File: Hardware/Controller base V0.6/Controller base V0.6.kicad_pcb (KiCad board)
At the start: 2 copper layers, 30.1 x 48.9 mm, 23 parts, among them J1 USB_C_Receptacle_USB2.0_16P, J7 Conn_02x10_Counter_Clockwise, J8 Conn_02x10_Counter_Clockwise, SW4 SW_Push, U1 AZ1117CH-3.3TRG1, U2 ESP32-S3-WROOM-1U-N4

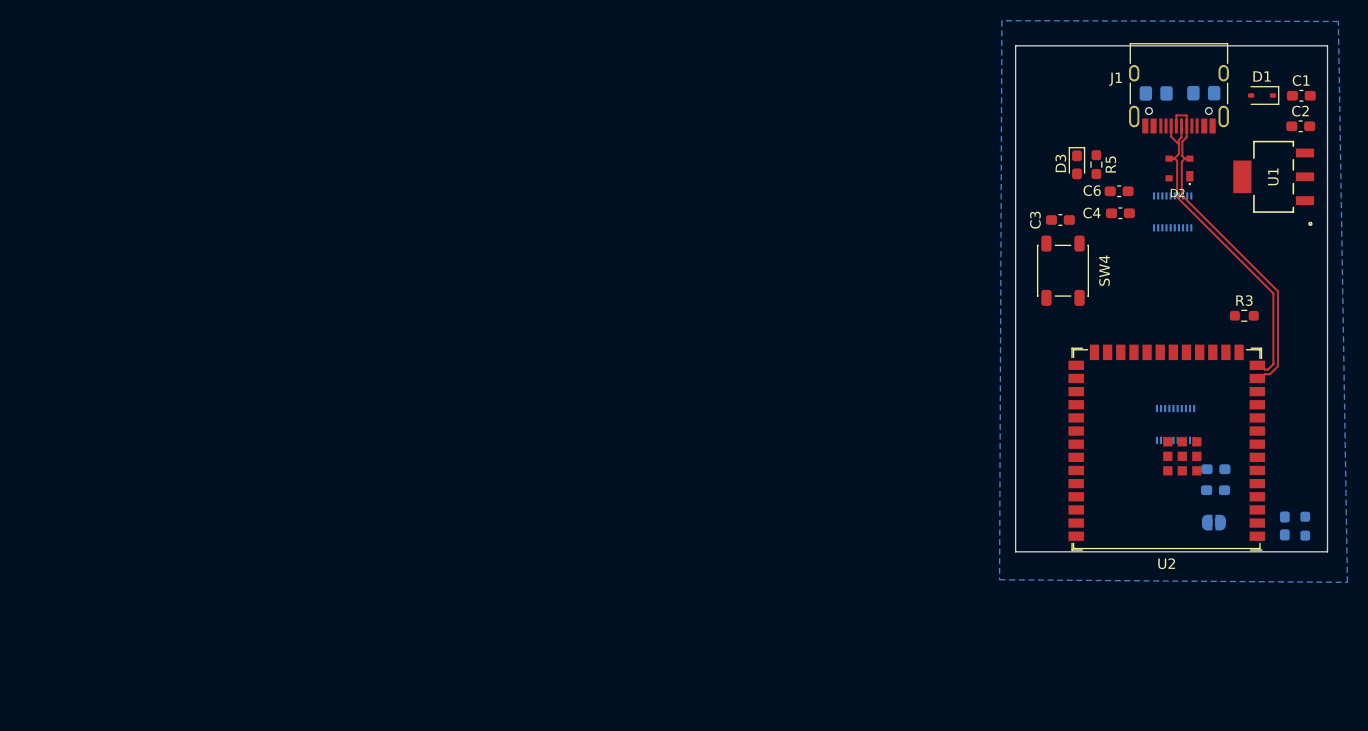
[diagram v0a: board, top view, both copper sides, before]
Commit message: .6 done
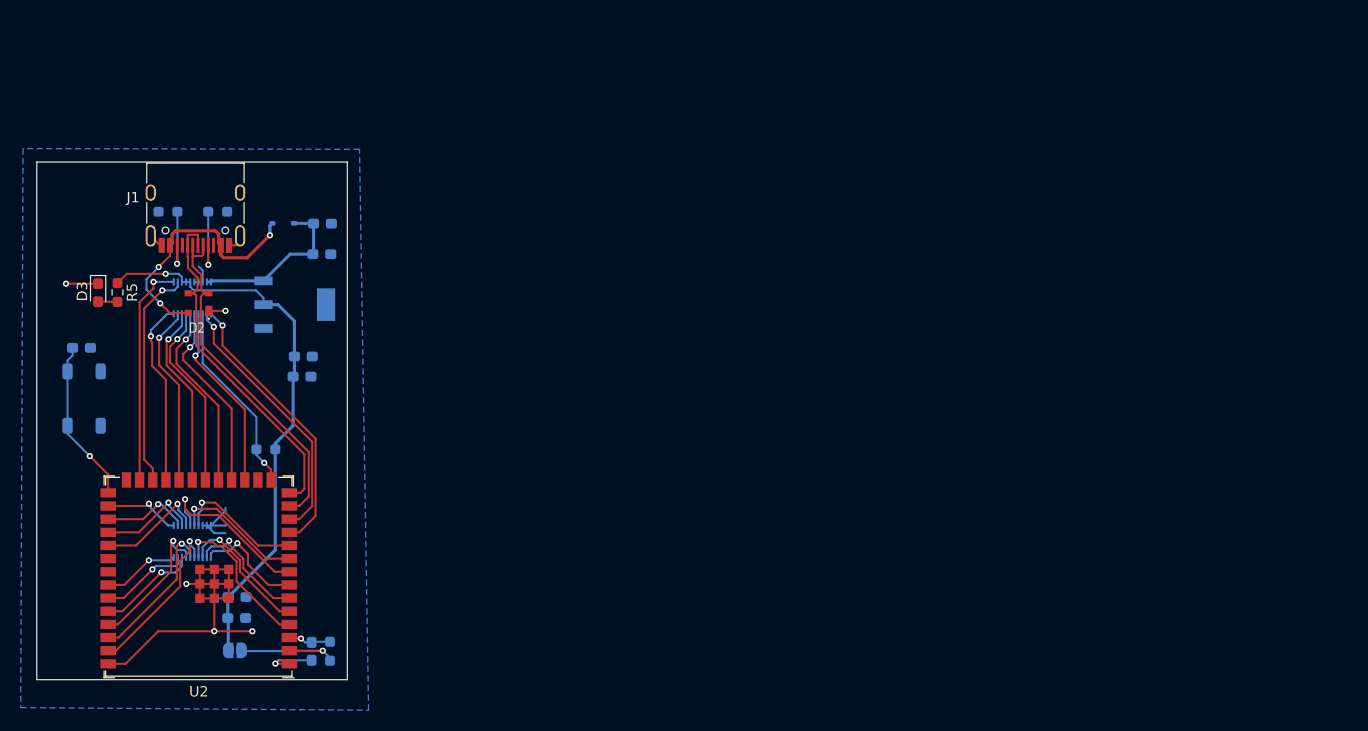
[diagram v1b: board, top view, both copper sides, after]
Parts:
- C1, C2, C3, C4, C6, D1, R3, SW4, U1: moved to B.Cu
- R1, R2: footprint Resistor_SMD:R_0805_2012Metric_Pad1.20x1.40mm_HandSolder -> Resistor_SMD:R_0603_1608Metric_Pad0.98x0.95mm_HandSolder
- moved R1 96.1 mm to (140.6, 73.7)
- moved R2 95.9 mm to (145.4, 73.7)
- moved J1 95.7 mm to (143.2, 72.9)
- moved J8 95.6 mm to (142.9, 105.5)
- moved D2 95.6 mm to (143.6, 82.5)
- moved R3 95.4 mm to (150.1, 96.6)
- moved C3 95.4 mm to (132.2, 86.8)
- moved D1 95.4 mm to (151.7, 74.8)
- moved D3 95.4 mm to (133.8, 81.5)
- moved R5 95.4 mm to (135.7, 81.5)
- moved R6 95.4 mm to (147.1, 116.0)
- moved SW4 95.4 mm to (132.5, 91.7), turned to 90 degrees
- moved U1 95.4 mm to (152.8, 82.6)
- moved C1 95.4 mm to (155.5, 74.8)
- moved C2 95.4 mm to (155.5, 77.8)
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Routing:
- net GND: track 0.00 -> 58.4 mm, vias 0 -> 6
- net VCC_3V3: track 0.00 -> 54.8 mm, vias 0 -> 1
- net GPIO18: track 0.00 -> 26.9 mm, vias 0 -> 1
- net GPIO8: track 0.00 -> 25.5 mm, vias 0 -> 1
- net VBUS: track 0.00 -> 25.2 mm, vias 0 -> 3
- net GPIO48: track 0.00 -> 21.6 mm, vias 0 -> 1
- net GPIO47: track 0.00 -> 21.6 mm, vias 0 -> 1
- net GPIO3: track 0.00 -> 18.8 mm, vias 0 -> 1
- net GPIO10: track 0.00 -> 18.4 mm, vias 0 -> 1
- net GPIO11: track 0.00 -> 18.3 mm, vias 0 -> 1
- net GPIO9: track 0.00 -> 18.1 mm, vias 0 -> 1
- net GPIO12: track 0.00 -> 18.1 mm, vias 0 -> 1
- net GPIO21: track 0.00 -> 17.9 mm, vias 0 -> 1
- net GPIO13: track 0.00 -> 17.7 mm, vias 0 -> 1
- net GPIO14: track 0.00 -> 17.6 mm, vias 0 -> 1
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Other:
- board size 30.1 x 48.9 mm -> 30 x 50 mm

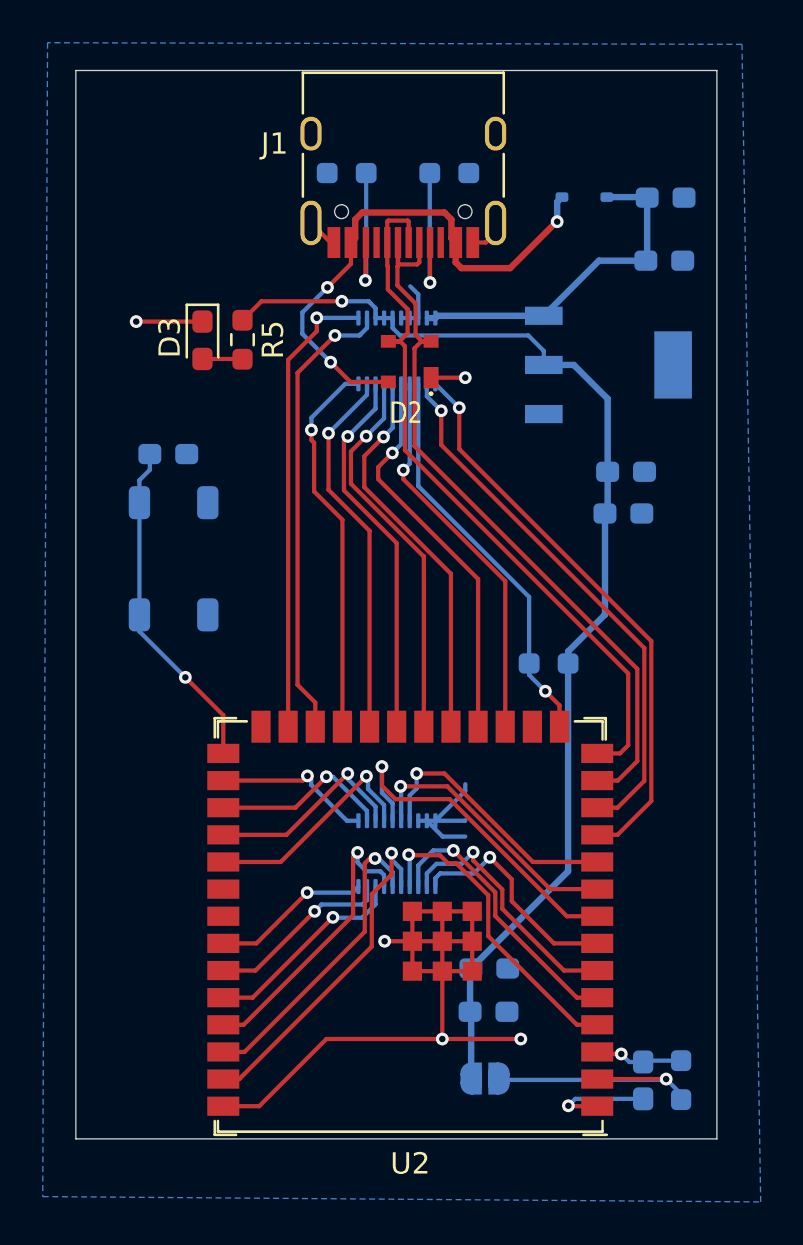
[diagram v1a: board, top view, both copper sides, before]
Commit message: updated carrier board
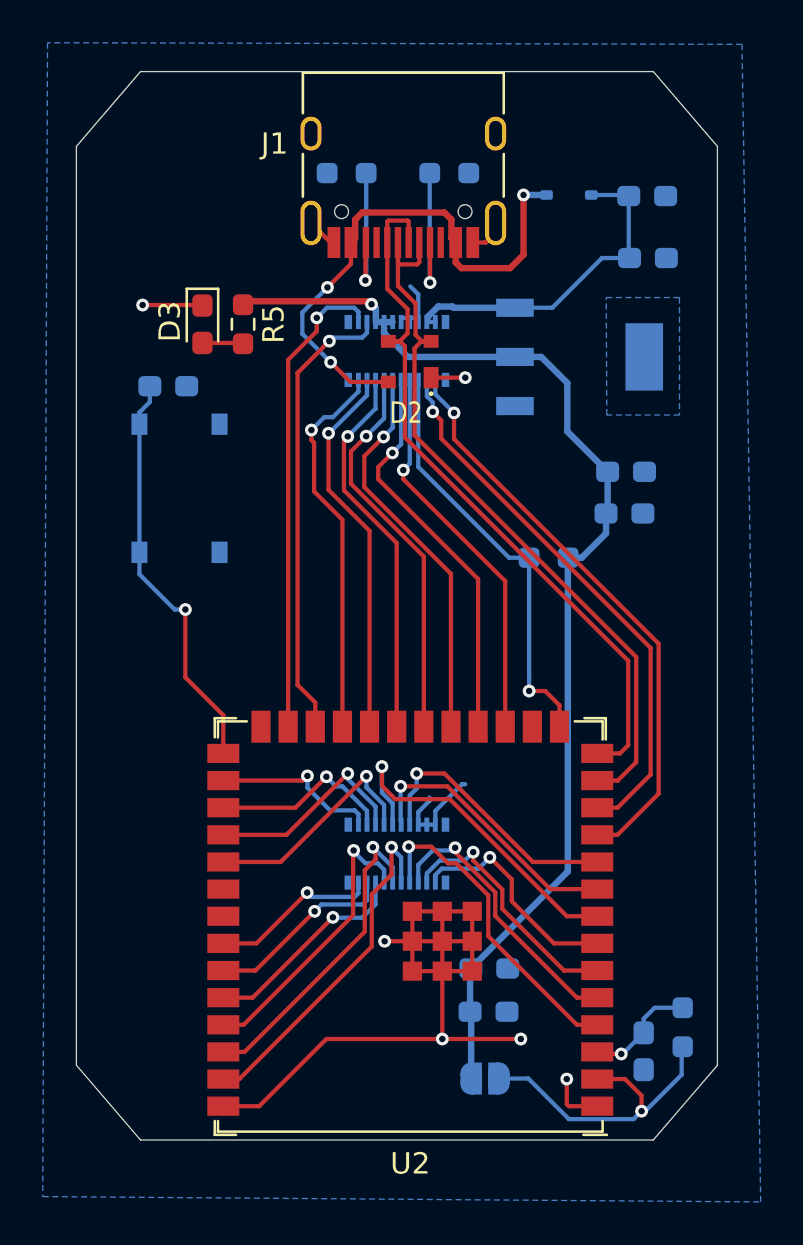
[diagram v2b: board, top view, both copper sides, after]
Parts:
- J7, J8: footprint Connector_Hirose_DF40:Hirose_DF40C-20DS-0.4V_2x10_P0.4mm -> DF40C:HRS_DF40C-20DP-0.4V_51_
- SW4: footprint Button_Switch_SMD:SW_SPST_PTS647_Sx38 -> Button_Switch_SMD:SW_Push_1P1T_XKB_TS-1187A
- moved R3 4.95 mm to (150.1, 91.7)
- moved SW4 3.31 mm to (132.8, 88.4)
- moved C3 3.17 mm to (132.2, 83.6)
- moved R4 2.48 mm to (156.3, 113.6)
- moved U1 1.40 mm to (151.5, 82.3)
- moved C8 1.36 mm to (154.5, 114.8)
- moved C1 0.87 mm to (154.7, 74.7)
- moved C2 0.77 mm to (154.7, 77.6)
- moved D3 0.75 mm to (133.8, 80.7)
- moved D1 0.73 mm to (151.0, 74.7)
- moved R5 0.73 mm to (135.8, 80.7)
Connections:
- J7 pad 1: GPIO48 -> GPIO21
- J7 pad 10: GPIO11 -> VCC_3V3
- J7 pad 11: GND -> GPIO10
- J7 pad 12: GPIO10 -> GND
- J7 pad 13: GND -> GPIO9
- J7 pad 14: GPIO9 -> GND
- J7 pad 15: GND -> GPIO3
- J7 pad 16: GPIO3 -> GND
- J7 pad 17: VCC_5V -> GPIO8
- J7 pad 18: GPIO8 -> VCC_5V
- J7 pad 19: VCC_5V -> GPIO18
- J7 pad 2: GPIO21 -> GPIO48
- J7 pad 20: GPIO18 -> VCC_5V
- J7 pad 3: GPIO47 -> GPIO14
- J7 pad 4: GPIO14 -> GPIO47
- J7 pad 5: VCC_3V3 -> GPIO13
- J7 pad 6: GPIO13 -> VCC_3V3
- J7 pad 7: VCC_3V3 -> GPIO12
- J7 pad 8: GPIO12 -> VCC_3V3
- J7 pad 9: VCC_3V3 -> GPIO11
- J8 pad 1: GPIO35 -> GPIO41
- J8 pad 10: GPIO2 -> GPIO15
- J8 pad 11: GPIO16 -> GPIO1
- J8 pad 12: GPIO1 -> GPIO16
- J8 pad 13: GPIO17 -> GPIO4
- J8 pad 14: GPIO4 -> GPIO17
- J8 pad 15: GND -> GPIO5
- J8 pad 16: GPIO5 -> GND
- J8 pad 17: GND -> GPIO6
- J8 pad 18: GPIO6 -> GND
- J8 pad 19: GND -> GPIO7
- J8 pad 2: GPIO41 -> GPIO35
- J8 pad 20: GPIO7 -> GND
- J8 pad 3: GPIO36 -> GPIO42
- J8 pad 4: GPIO42 -> GPIO36
- J8 pad 5: GPIO37 -> RXD0
- J8 pad 6: RXD0 -> GPIO37
- J8 pad 7: GPIO38 -> TXD0
- J8 pad 8: TXD0 -> GPIO38
- J8 pad 9: GPIO15 -> GPIO2
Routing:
- net GND: track 58.4 -> 53.6 mm
- net GPIO0: track 15.8 -> 19.3 mm
- net ESP_3.3V: track 13.2 -> 15.3 mm
- net GPIO3: track 18.8 -> 19.8 mm
- net GPIO2: track 14.5 -> 15.4 mm
- net /CHIP_PU: track 4.49 -> 5.32 mm
- net GPIO4: track 14.8 -> 15.5 mm
- net GPIO41: track 7.43 -> 8.14 mm
- net GPIO48: track 21.6 -> 22.2 mm
- net GPIO1: track 16.0 -> 16.6 mm
- added copper zone on B.Cu, net unconnected-(U1-EPAD-Pad4)
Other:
- outline, holes or cut-outs redrawn
